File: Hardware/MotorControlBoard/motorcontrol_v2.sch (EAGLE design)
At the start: 27 parts, among them U1 ATMEGA328P-AU

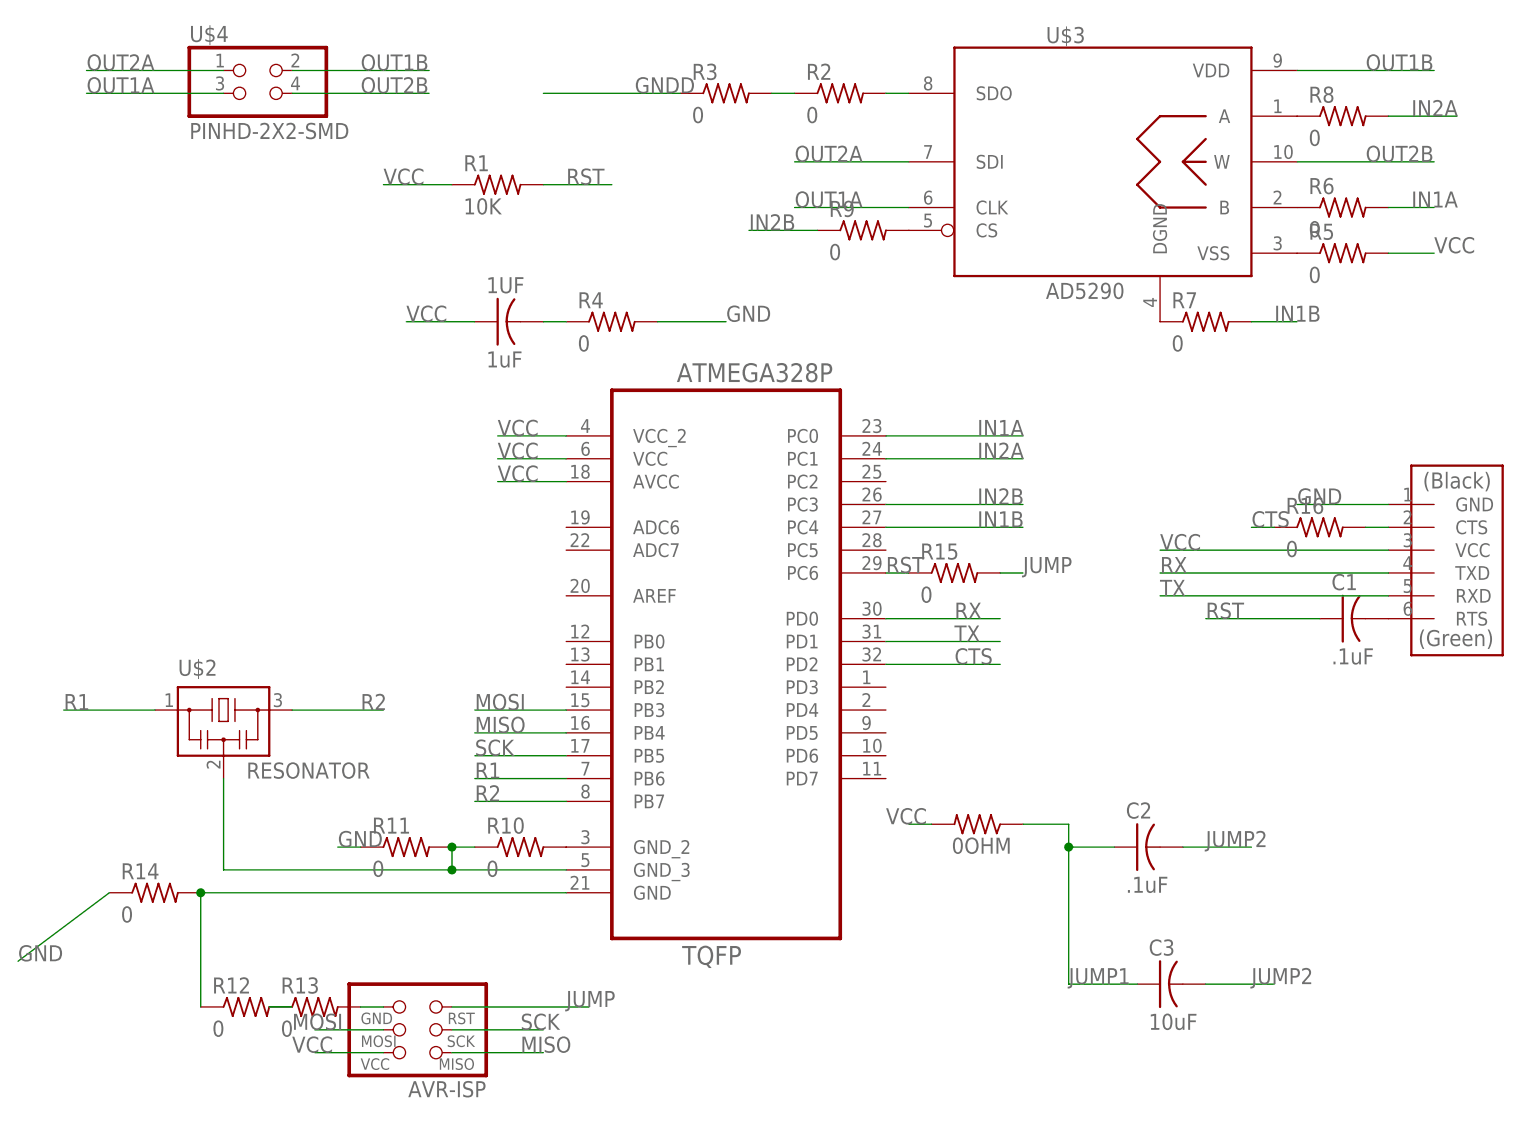
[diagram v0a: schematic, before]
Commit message: new case
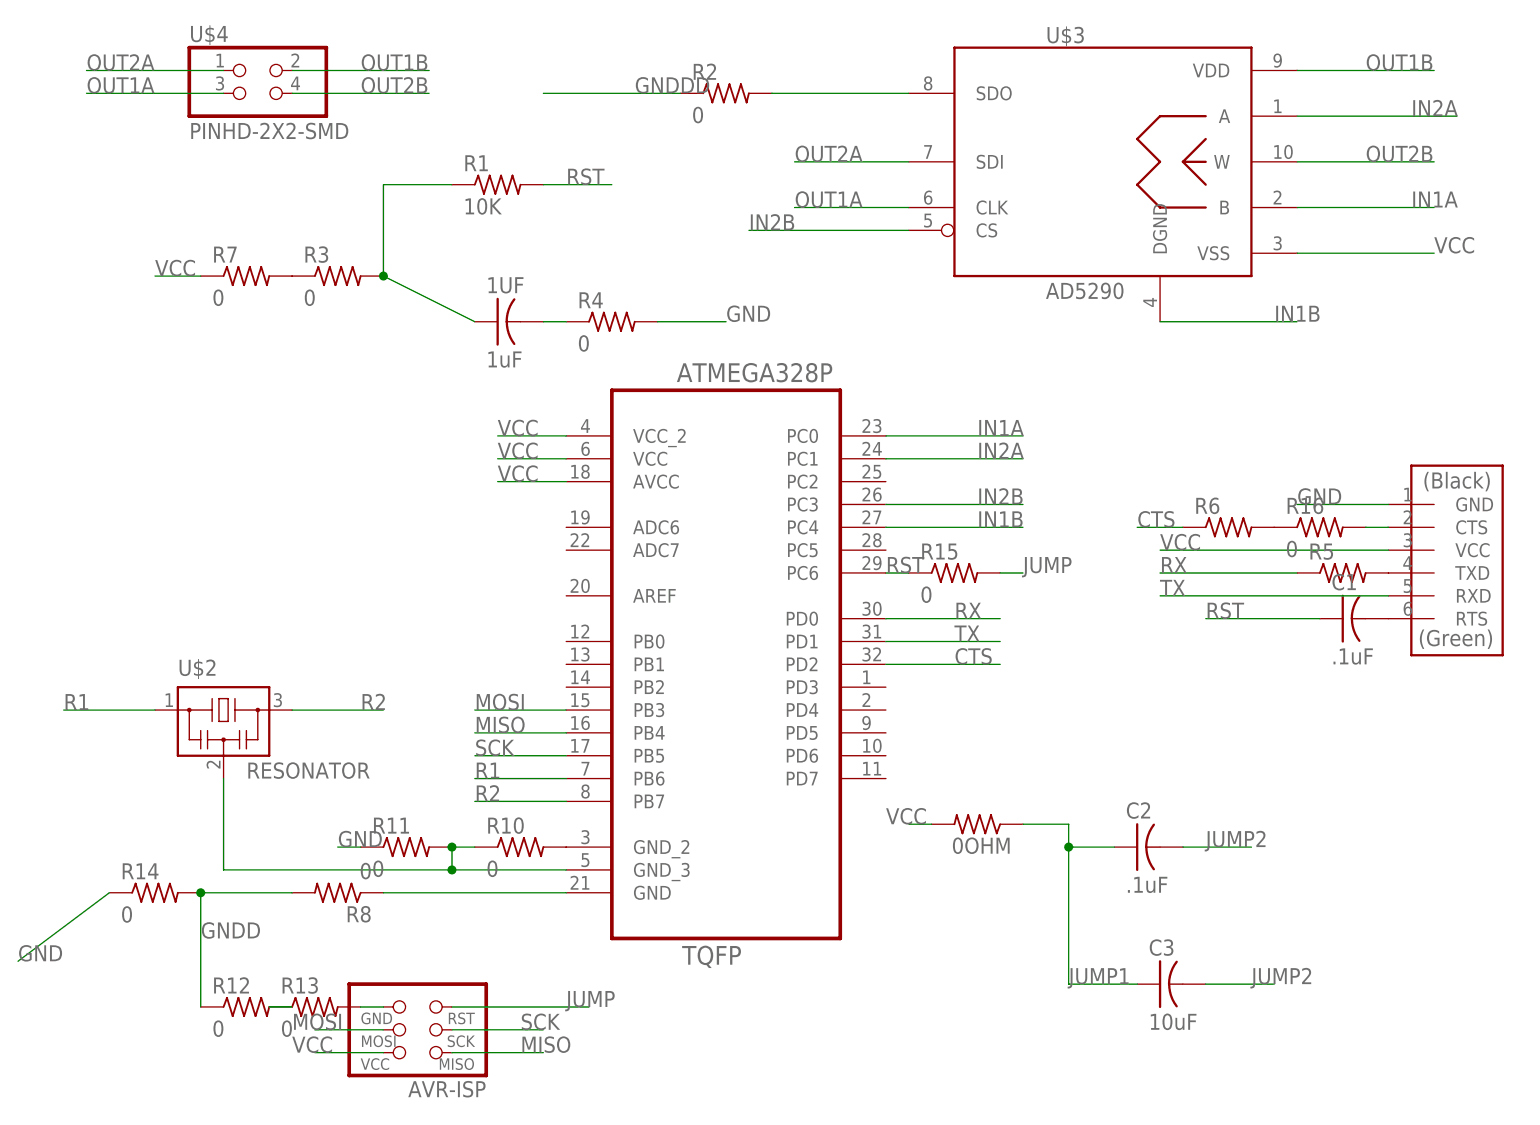
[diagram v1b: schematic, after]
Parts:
- removed R9: 0, fab:RES-US1206
- R5: value 0 -> (none)
- R6: value 0 -> (none); device fab:RES-US1206 -> fab:RES-US1206FAB
- R7, R8: device fab:RES-US1206 -> fab:RES-US1206FAB
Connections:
- removed net N$11: R2.1, R3.2
- removed net N$5: R9.2, U$3.CS
- new net GNDDD: R2.1, R8.1, U1.GND
- net CTS: now also R6.1; no longer R16.1
- net GNDD: now also R8.2; no longer R3.1, U1.GND
- net IN1A: now also U$3.B; no longer R6.2
- net IN1B: now also U$3.DGND; no longer R7.2
- net IN2A: now also U$3.A; no longer R8.2
- net IN2B: now also U$3.CS; no longer R9.1
- net N$1: now also R5.2, U$1.TXD; no longer R5.1, U$3.VSS
- net N$2: now also R16.1, R6.2; no longer R6.1, U$3.B
- net N$3: now also 1UF.1, R1.1, R3.2; no longer R7.1, U$3.DGND
- net N$4: now also R3.1, R7.2; no longer R8.1, U$3.A
- net RX: now also R5.1; no longer U$1.TXD
- net VCC: now also R7.1, U$3.VSS; no longer 1UF.1, R1.1, R5.2
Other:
- moved on the sheet: R2, R3, R5, R6, R7, R8
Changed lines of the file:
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@@
 <part name="0OHM" library="fab" deviceset="RES-US" device="1206FAB"/>
 <part name="R2" library="fab" deviceset="RES-US" device="1206FAB" value="0"/>
-<part name="R3" library="fab" deviceset="RES-US" device="1206FAB" value="0"/>
 <part name="R4" library="fab" deviceset="RES-US" device="1206FAB" value="0"/>
 <part name="R10" library="fab" deviceset="RES-US" device="1206FAB" value="0"/>
@@
 <part name="R13" library="fab" deviceset="RES-US" device="1206" value="0"/>
 <part name="R15" library="fab" deviceset="RES-US" device="1206FAB" value="0"/>
-<part name="R5" library="fab" deviceset="RES-US" device="1206FAB" value="0"/>
-<part name="R6" library="fab" deviceset="RES-US" device="1206" value="0"/>
-<part name="R7" library="fab" deviceset="RES-US" device="1206" value="0"/>
-<part name="R8" library="fab" deviceset="RES-US" device="1206" value="0"/>
-<part name="R9" library="fab" deviceset="RES-US" device="1206" value="0"/>
 <part name="R14" library="fab" deviceset="RES-US" device="1206FAB" value="0"/>
 <part name="R16" library="fab" deviceset="RES-US" device="1206FAB" value="0"/>
 <part name="C1" library="fab" deviceset="CAP-US" device="1206FAB" value=".1uF"/>
+<part name="R5" library="fab" deviceset="RES-US" device="1206FAB"/>
+<part name="R6" library="fab" deviceset="RES-US" device="1206FAB"/>
+<part name="R3" library="fab" deviceset="RES-US" device="1206FAB" value="0"/>
+<part name="R7" library="fab" deviceset="RES-US" device="1206FAB" value="0"/>
+<part name="R8" library="fab" deviceset="RES-US" device="1206FAB" value="0"/>
 </parts>
 <sheets>
@@
 <instance part="U$4" gate="G$1" x="25.4" y="114.3"/>
 <instance part="0OHM" gate="G$1" x="104.14" y="33.02" rot="R180"/>
-<instance part="R2" gate="G$1" x="88.9" y="114.3"/>
-<instance part="R3" gate="G$1" x="76.2" y="114.3"/>
+<instance part="R2" gate="G$1" x="76.2" y="114.3"/>
 <instance part="R4" gate="G$1" x="63.5" y="88.9"/>
 <instance part="R10" gate="G$1" x="53.34" y="30.48"/>
@@
 <instance part="R13" gate="G$1" x="30.48" y="12.7"/>
 <instance part="R15" gate="G$1" x="101.6" y="60.96"/>
-<instance part="R5" gate="G$1" x="144.78" y="96.52"/>
-<instance part="R6" gate="G$1" x="144.78" y="101.6"/>
-<instance part="R7" gate="G$1" x="129.54" y="88.9"/>
-<instance part="R8" gate="G$1" x="144.78" y="111.76"/>
-<instance part="R9" gate="G$1" x="91.44" y="99.06"/>
 <instance part="R14" gate="G$1" x="12.7" y="25.4"/>
 <instance part="R16" gate="G$1" x="142.24" y="66.04"/>
 <instance part="C1" gate="G$1" x="144.78" y="55.88"/>
+<instance part="R5" gate="G$1" x="144.78" y="60.96"/>
+<instance part="R6" gate="G$1" x="132.08" y="66.04"/>
+<instance part="R3" gate="G$1" x="33.02" y="93.98"/>
+<instance part="R7" gate="G$1" x="22.86" y="93.98"/>
+<instance part="R8" gate="G$1" x="33.02" y="25.4" rot="R180"/>
 </instances>
 <busses>
@@
 <net name="VCC" class="0">
 <segment>
-<pinref part="R1" gate="G$1" pin="1"/>
-<wire x1="45.72" y1="104.14" x2="38.1" y2="104.14" width="0.1524" layer="91"/>
-<label x="38.1" y="104.14" size="1.778" layer="95"/>
-</segment>
-<segment>
-<pinref part="1UF" gate="G$1" pin="1"/>
-<wire x1="48.26" y1="88.9" x2="40.64" y2="88.9" width="0.1524" layer="91"/>
-<label x="40.64" y="88.9" size="1.778" layer="95"/>
-</segment>
-<segment>
 <pinref part="U1" gate="A" pin="VCC"/>
 <wire x1="58.42" y1="73.66" x2="50.8" y2="73.66" width="0.1524" layer="91"/>
@@
 </segment>
 <segment>
-<pinref part="R5" gate="G$1" pin="2"/>
-<wire x1="149.86" y1="96.52" x2="154.94" y2="96.52" width="0.1524" layer="91"/>
 <label x="154.94" y="96.52" size="1.778" layer="95"/>
+<pinref part="U$3" gate="G$1" pin="VSS"/>
+<wire x1="139.7" y1="96.52" x2="154.94" y2="96.52" width="0.1524" layer="91"/>
 </segment>
 <segment>
@@
 <wire x1="38.1" y1="7.62" x2="30.48" y2="7.62" width="0.1524" layer="91"/>
 <label x="27.94" y="7.62" size="1.778" layer="95"/>
+</segment>
+<segment>
+<pinref part="R7" gate="G$1" pin="1"/>
+<wire x1="17.78" y1="93.98" x2="12.7" y2="93.98" width="0.1524" layer="91"/>
+<label x="12.7" y="93.98" size="1.778" layer="95"/>
 </segment>
 </net>
@@
 </segment>
 <segment>
-<pinref part="U$1" gate="G$1" pin="TXD"/>
-<wire x1="149.86" y1="60.96" x2="124.46" y2="60.96" width="0.1524" layer="91"/>
+<pinref part="R5" gate="G$1" pin="1"/>
+<wire x1="139.7" y1="60.96" x2="124.46" y2="60.96" width="0.1524" layer="91"/>
 <label x="124.46" y="60.96" size="1.778" layer="95"/>
 </segment>
@@
 </segment>
 <segment>
-<pinref part="R9" gate="G$1" pin="1"/>
-<wire x1="86.36" y1="99.06" x2="78.74" y2="99.06" width="0.1524" layer="91"/>
 <label x="78.74" y="99.06" size="1.778" layer="95"/>
+<pinref part="U$3" gate="G$1" pin="CS"/>
+<wire x1="96.52" y1="99.06" x2="78.74" y2="99.06" width="0.1524" layer="91"/>
 </segment>
 </net>
@@
 </segment>
 <segment>
-<pinref part="R8" gate="G$1" pin="2"/>
-<wire x1="149.86" y1="111.76" x2="157.48" y2="111.76" width="0.1524" layer="91"/>
 <label x="152.4" y="111.76" size="1.778" layer="95"/>
+<pinref part="U$3" gate="G$1" pin="A"/>
+<wire x1="157.48" y1="111.76" x2="139.7" y2="111.76" width="0.1524" layer="91"/>
 </segment>
 </net>
@@
 </segment>
 <segment>
-<pinref part="R6" gate="G$1" pin="2"/>
-<wire x1="149.86" y1="101.6" x2="154.94" y2="101.6" width="0.1524" layer="91"/>
 <label x="152.4" y="101.6" size="1.778" layer="95"/>
+<pinref part="U$3" gate="G$1" pin="B"/>
+<wire x1="154.94" y1="101.6" x2="139.7" y2="101.6" width="0.1524" layer="91"/>
 </segment>
 </net>
@@
 </segment>
 <segment>
-<pinref part="R7" gate="G$1" pin="2"/>
-<wire x1="134.62" y1="88.9" x2="139.7" y2="88.9" width="0.1524" layer="91"/>
 <label x="137.16" y="88.9" size="1.778" layer="95"/>
+<pinref part="U$3" gate="G$1" pin="DGND"/>
+<wire x1="124.46" y1="88.9" x2="139.7" y2="88.9" width="0.1524" layer="91"/>
 </segment>
 </net>
@@
 <pinref part="U$3" gate="G$1" pin="SDO"/>
 <pinref part="R2" gate="G$1" pin="2"/>
-<wire x1="93.98" y1="114.3" x2="96.52" y2="114.3" width="0.1524" layer="91"/>
+<wire x1="81.28" y1="114.3" x2="96.52" y2="114.3" width="0.1524" layer="91"/>
 </segment>
 </net>
@@
 <pinref part="U1" gate="A" pin="GND_2"/>
 <pinref part="R10" gate="G$1" pin="2"/>
-</segment>
-</net>
-<net name="N$1" class="0">
-<segment>
-<pinref part="U$3" gate="G$1" pin="VSS"/>
-<pinref part="R5" gate="G$1" pin="1"/>
-</segment>
-</net>
-<net name="N$2" class="0">
-<segment>
-<pinref part="U$3" gate="G$1" pin="B"/>
-<pinref part="R6" gate="G$1" pin="1"/>
-</segment>
-</net>
-<net name="N$3" class="0">
-<segment>
-<pinref part="U$3" gate="G$1" pin="DGND"/>
-<pinref part="R7" gate="G$1" pin="1"/>
-</segment>
-</net>
-<net name="N$4" class="0">
-<segment>
-<pinref part="U$3" gate="G$1" pin="A"/>
-<pinref part="R8" gate="G$1" pin="1"/>
-</segment>
-</net>
-<net name="N$5" class="0">
-<segment>
-<pinref part="U$3" gate="G$1" pin="CS"/>
-<pinref part="R9" gate="G$1" pin="2"/>
-</segment>
-</net>
-<net name="N$11" class="0">
-<segment>
-<pinref part="R2" gate="G$1" pin="1"/>
-<pinref part="R3" gate="G$1" pin="2"/>
-<wire x1="81.28" y1="114.3" x2="83.82" y2="114.3" width="0.1524" layer="91"/>
 </segment>
 </net>
@@
 <net name="GNDD" class="0">
 <segment>
-<pinref part="R3" gate="G$1" pin="1"/>
-<wire x1="71.12" y1="114.3" x2="55.88" y2="114.3" width="0.1524" layer="91"/>
-<label x="66.04" y="114.3" size="1.778" layer="95"/>
-</segment>
-<segment>
+<pinref part="R14" gate="G$1" pin="2"/>
 <pinref part="R12" gate="G$1" pin="1"/>
 <wire x1="17.78" y1="12.7" x2="17.78" y2="25.4" width="0.1524" layer="91"/>
-<pinref part="U1" gate="A" pin="GND"/>
-<wire x1="17.78" y1="25.4" x2="58.42" y2="25.4" width="0.1524" layer="91"/>
-<pinref part="R14" gate="G$1" pin="2"/>
+<pinref part="R8" gate="G$1" pin="2"/>
+<wire x1="27.94" y1="25.4" x2="17.78" y2="25.4" width="0.1524" layer="91"/>
 <junction x="17.78" y="25.4"/>
+<label x="17.78" y="20.32" size="1.778" layer="95"/>
 </segment>
 </net>
@@
 </segment>
 <segment>
-<pinref part="R16" gate="G$1" pin="1"/>
-<wire x1="137.16" y1="66.04" x2="134.62" y2="66.04" width="0.1524" layer="91"/>
-<label x="134.62" y="66.04" size="1.778" layer="95"/>
+<pinref part="R6" gate="G$1" pin="1"/>
+<wire x1="127" y1="66.04" x2="121.92" y2="66.04" width="0.1524" layer="91"/>
+<label x="121.92" y="66.04" size="1.778" layer="95"/>
 </segment>
 </net>
@@
 </segment>
 </net>
+<net name="N$1" class="0">
+<segment>
+<pinref part="U$1" gate="G$1" pin="TXD"/>
+<pinref part="R5" gate="G$1" pin="2"/>
+</segment>
+</net>
+<net name="N$2" class="0">
+<segment>
+<pinref part="R16" gate="G$1" pin="1"/>
+<pinref part="R6" gate="G$1" pin="2"/>
+</segment>
+</net>
+<net name="N$3" class="0">
+<segment>
+<pinref part="1UF" gate="G$1" pin="1"/>
+<pinref part="R3" gate="G$1" pin="2"/>
+<wire x1="38.1" y1="93.98" x2="48.26" y2="88.9" width="0.1524" layer="91"/>
+<pinref part="R1" gate="G$1" pin="1"/>
+<wire x1="45.72" y1="104.14" x2="38.1" y2="104.14" width="0.1524" layer="91"/>
+<wire x1="38.1" y1="104.14" x2="38.1" y2="93.98" width="0.1524" layer="91"/>
+<junction x="38.1" y="93.98"/>
+</segment>
+</net>
+<net name="N$4" class="0">
+<segment>
+<pinref part="R3" gate="G$1" pin="1"/>
+<pinref part="R7" gate="G$1" pin="2"/>
+</segment>
+</net>
+<net name="GNDDD" class="0">
+<segment>
+<wire x1="71.12" y1="114.3" x2="55.88" y2="114.3" width="0.1524" layer="91"/>
+<label x="66.04" y="114.3" size="1.778" layer="95"/>
+<pinref part="R2" gate="G$1" pin="1"/>
+</segment>
+<segment>
+<pinref part="U1" gate="A" pin="GND"/>
+<pinref part="R8" gate="G$1" pin="1"/>
+<wire x1="58.42" y1="25.4" x2="38.1" y2="25.4" width="0.1524" layer="91"/>
+</segment>
+</net>
